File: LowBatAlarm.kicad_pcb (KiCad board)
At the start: 2 copper layers, 30 x 24 mm, 19 parts, among them J1 Battery, J2 Buzzer, Q1 BSN20, U1 ADCMP350, U2 ADP7142AUJZ

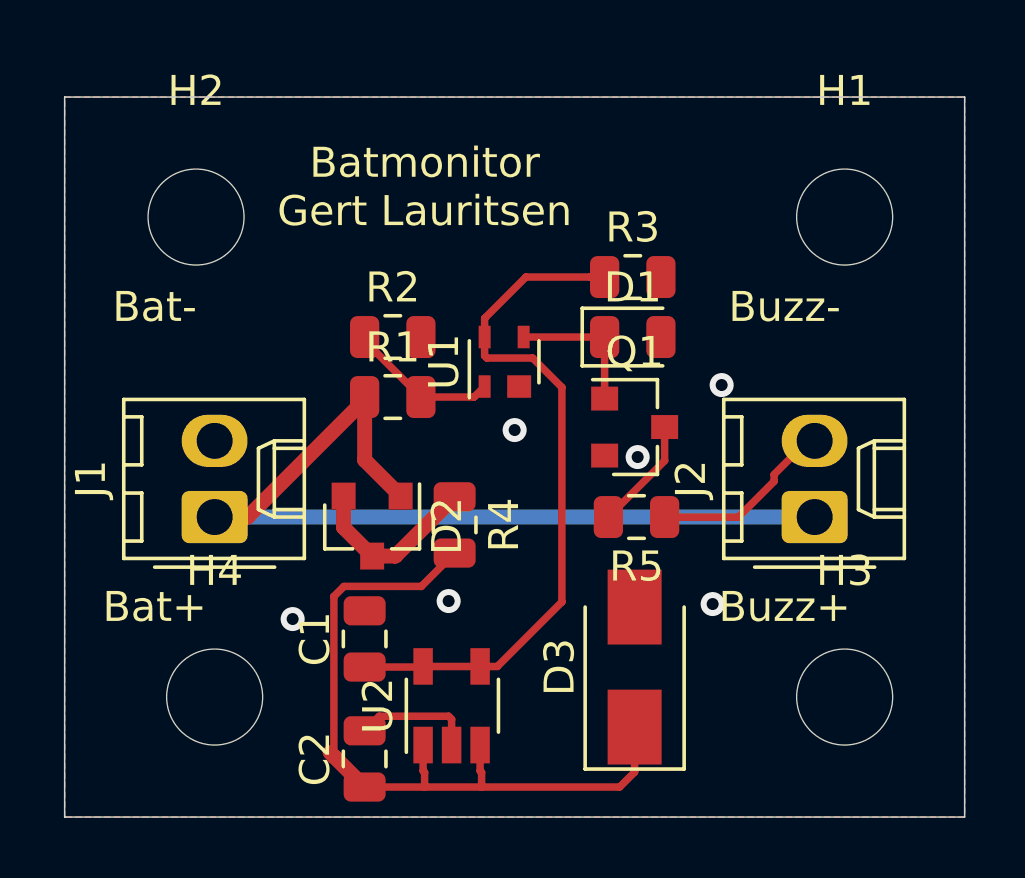
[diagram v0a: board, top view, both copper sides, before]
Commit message: PCB opdatering
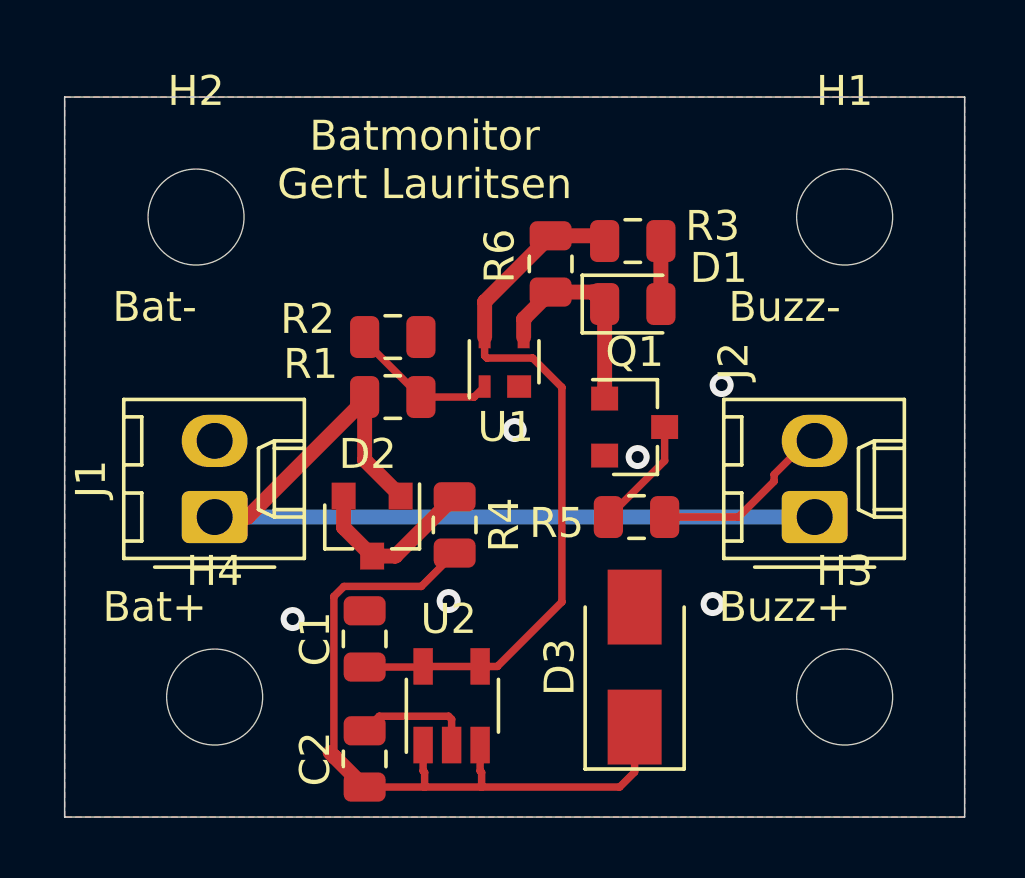
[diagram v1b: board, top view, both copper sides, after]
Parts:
- added R6: 1k, Resistor_SMD:R_0805_2012Metric, F.Cu at (140.2, 91.6)
- R2: value 100k -> TBD
- moved R3 1.20 mm to (142.9, 90.8)
- moved D1 1.10 mm to (142.9, 92.9)
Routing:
- net Net-(D1-Pad1): track 4.75 -> 6.99 mm
- net Net-(D1-Pad2): track 0.00 -> 2.10 mm
- net +3V3: track 23.5 -> 24.4 mm
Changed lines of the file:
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@@
     (thickness 1.6)
     (drawings 11)
-    (tracks 66)
+    (tracks 70)
     (zones 0)
-    (modules 19)
+    (modules 20)
     (nets 11)
   )
@@
   )
   (setup
-    (last_trace_width 0.25)
+    (last_trace_width 0.5)
     (user_trace_width 0.5)
     (trace_clearance 0.2)
@@
     (solder_mask_min_width 0.25)
     (aux_axis_origin 0 0)
-    (visible_elements 7FFFFFFF)
+    (visible_elements 7FF9FFFF)
     (pcbplotparams
       (layerselection 0x010fc_ffffffff)
@@
   )
   (module Resistor_SMD:R_0805_2012Metric (layer F.Cu)
+    (at 140.2 91.5625 270)
+    (descr "Resistor SMD 0805 (2012 Metric), square (rectangular) end terminal, IPC_7351 nominal, (Body size source: https://docs.google.com/spreadsheets/d/1BsfQQcO9C6DZCsRaXUlFlo91Tg2WpOkGARC1WS5S8t0/edit?usp=sharing), generated with kicad-footprint-generator")
+    (tags resistor)
+    (attr smd)
+    (fp_text reference R6 (at -0.2625 1.7 90) (layer F.SilkS)
+      (effects (font (size 1 1) (thickness 0.15)))
+    )
+    (fp_text value 1k (at 0 1.65 90) (layer F.Fab)
+      (effects (font (size 1 1) (thickness 0.15)))
+    )
+    (fp_text user %R (at 0 0 90) (layer F.Fab)
+      (effects (font (size 0.5 0.5) (thickness 0.08)))
+    )
+    (fp_line (start 1.68 0.95) (end -1.68 0.95) (layer F.CrtYd) (width 0.05))
+    (fp_line (start 1.68 -0.95) (end 1.68 0.95) (layer F.CrtYd) (width 0.05))
+    (fp_line (start -1.68 -0.95) (end 1.68 -0.95) (layer F.CrtYd) (width 0.05))
+    (fp_line (start -1.68 0.95) (end -1.68 -0.95) (layer F.CrtYd) (width 0.05))
+    (fp_line (start -0.258578 0.71) (end 0.258578 0.71) (layer F.SilkS) (width 0.12))
+    (fp_line (start -0.258578 -0.71) (end 0.258578 -0.71) (layer F.SilkS) (width 0.12))
+    (fp_line (start 1 0.6) (end -1 0.6) (layer F.Fab) (width 0.1))
+    (fp_line (start 1 -0.6) (end 1 0.6) (layer F.Fab) (width 0.1))
+    (fp_line (start -1 -0.6) (end 1 -0.6) (layer F.Fab) (width 0.1))
+    (fp_line (start -1 0.6) (end -1 -0.6) (layer F.Fab) (width 0.1))
+    (pad 2 smd roundrect (at 0.9375 0 270) (size 0.975 1.4) (layers F.Cu F.Paste F.Mask) (roundrect_rratio 0.25)
+      (net 2 "Net-(D1-Pad1)"))
+    (pad 1 smd roundrect (at -0.9375 0 270) (size 0.975 1.4) (layers F.Cu F.Paste F.Mask) (roundrect_rratio 0.25)
+      (net 7 +3V3))
+    (model ${KISYS3DMOD}/Resistor_SMD.3dshapes/R_0805_2012Metric.wrl
+      (at (xyz 0 0 0))
+      (scale (xyz 1 1 1))
+      (rotate (xyz 0 0 0))
+    )
+  )
+  (module Resistor_SMD:R_0805_2012Metric (layer F.Cu)
     (at 143.0625 100 180)
     (descr "Resistor SMD 0805 (2012 Metric), square (rectangular) end terminal, IPC_7351 nominal, (Body size source: https://docs.google.com/spreadsheets/d/1BsfQQcO9C6DZCsRaXUlFlo91Tg2WpOkGARC1WS5S8t0/edit?usp=sharing), generated with kicad-footprint-generator")
     (tags resistor)
     (attr smd)
-    (fp_text reference R5 (at 0 -1.65) (layer F.SilkS)
+    (fp_text reference R5 (at 2.6625 -0.2) (layer F.SilkS)
       (effects (font (size 1 1) (thickness 0.15)))
     )
@@
     (tags SOT-23)
     (attr smd)
-    (fp_text reference D2 (at 0 -2.5 90) (layer F.SilkS)
+    (fp_text reference D2 (at -2.4 0.15 180) (layer F.SilkS)
       (effects (font (size 1 1) (thickness 0.15)))
     )
@@
     (tags TSOT-23-5)
     (attr smd)
-    (fp_text reference U2 (at 0 -2.45 90) (layer F.SilkS)
+    (fp_text reference U2 (at 2.89 -0.1 180) (layer F.SilkS)
       (effects (font (size 1 1) (thickness 0.15)))
     )
@@
     (tags resistor)
     (attr smd)
-    (fp_text reference R2 (at 0 -1.65) (layer F.SilkS)
-      (effects (font (size 1 1) (thickness 0.15)))
-    )
-    (fp_text value 100k (at 0 1.65) (layer F.Fab)
-      (effects (font (size 1 1) (thickness 0.15)))
-    )
-    (fp_text user %R (at 0 0) (layer F.Fab)
+    (fp_text reference R2 (at -2.8375 -0.6) (layer F.SilkS)
+      (effects (font (size 1 1) (thickness 0.15)))
+    )
+    (fp_text value TBD (at 0 1.65) (layer F.Fab)
+      (effects (font (size 1 1) (thickness 0.15)))
+    )
+    (fp_text user %R (at -2.6375 1.3) (layer F.Fab)
       (effects (font (size 0.5 0.5) (thickness 0.08)))
     )
@@
     (tags resistor)
     (attr smd)
-    (fp_text reference R1 (at 0 -1.65) (layer F.SilkS)
+    (fp_text reference R1 (at -2.7375 -1.1) (layer F.SilkS)
       (effects (font (size 1 1) (thickness 0.15)))
     )
@@
     (tags "Analog Devices KS-4 (like EIAJ SC-82)")
     (attr smd)
-    (fp_text reference U1 (at 0 -2 90) (layer F.SilkS)
+    (fp_text reference U1 (at -2.175 0.05 180) (layer F.SilkS)
       (effects (font (size 1 1) (thickness 0.15)))
     )
@@
   )
   (module Resistor_SMD:R_0805_2012Metric (layer F.Cu)
-    (at 142.9375 92)
+    (at 142.9375 90.8)
     (descr "Resistor SMD 0805 (2012 Metric), square (rectangular) end terminal, IPC_7351 nominal, (Body size source: https://docs.google.com/spreadsheets/d/1BsfQQcO9C6DZCsRaXUlFlo91Tg2WpOkGARC1WS5S8t0/edit?usp=sharing), generated with kicad-footprint-generator")
     (tags resistor)
     (attr smd)
-    (fp_text reference R3 (at 0 -1.65) (layer F.SilkS)
+    (fp_text reference R3 (at 2.6625 -0.5) (layer F.SilkS)
       (effects (font (size 1 1) (thickness 0.15)))
     )
@@
     (descr "Molex KK-254 Interconnect System, old/engineering part number: AE-6410-02A example for new part number: 22-27-2021, 2 Pins (http://www.molex.com/pdm_docs/sd/022272021_sd.pdf), generated with kicad-footprint-generator")
     (tags "connector Molex KK-254 side entry")
-    (fp_text reference J2 (at 1.27 -4.12 90) (layer F.SilkS)
+    (fp_text reference J2 (at 5.2 -2.7 90) (layer F.SilkS)
       (effects (font (size 1 1) (thickness 0.15)))
     )
@@
   )
   (module LED_SMD:LED_0805_2012Metric (layer F.Cu)
-    (at 142.9375 94)
+    (at 142.9375 92.9)
     (descr "LED SMD 0805 (2012 Metric), square (rectangular) end terminal, IPC_7351 nominal, (Body size source: https://docs.google.com/spreadsheets/d/1BsfQQcO9C6DZCsRaXUlFlo91Tg2WpOkGARC1WS5S8t0/edit?usp=sharing), generated with kicad-footprint-generator")
     (tags diode)
     (attr smd)
-    (fp_text reference D1 (at 0 -1.65) (layer F.SilkS)
+    (fp_text reference D1 (at 2.8625 -1.2) (layer F.SilkS)
       (effects (font (size 1 1) (thickness 0.15)))
     )
@@
     (effects (font (size 1 1) (thickness 0.15)))
   )
-  (gr_text "Batmonitor\nGert Lauritsen" (at 136 89) (layer F.SilkS)
+  (gr_text "Batmonitor\nGert Lauritsen" (at 136 88.1) (layer F.SilkS)
     (effects (font (size 1 1) (thickness 0.15)))
   )
@@
   (gr_line (start 154 86) (end 154 110) (layer Edge.Cuts) (width 0.05))
   (gr_line (start 124 86) (end 154 86) (layer Edge.Cuts) (width 0.05))
-  (segment (start 139.3 94) (end 142 94) (width 0.25) (layer F.Cu) (net 2))
-  (segment (start 142 96.05) (end 142 94) (width 0.25) (layer F.Cu) (net 2))
+  (segment (start 143.875 90.8) (end 143.875 92.9) (width 0.5) (layer F.Cu) (net 1))
+  (segment (start 141.6 92.5) (end 142 92.9) (width 0.5) (layer F.Cu) (net 2))
+  (segment (start 140.2 92.5) (end 141.6 92.5) (width 0.5) (layer F.Cu) (net 2))
+  (segment (start 139.3 93.4) (end 140.2 92.5) (width 0.5) (layer F.Cu) (net 2))
+  (segment (start 139.3 94) (end 139.3 93.4) (width 0.5) (layer F.Cu) (net 2))
+  (segment (start 142 96.05) (end 142 92.9) (width 0.5) (layer F.Cu) (net 2))
   (segment (start 136.799473 106.639473) (end 134.485527 106.639473) (width 0.25) (layer F.Cu) (net 3))
   (segment (start 134.485527 106.639473) (end 134 107.125) (width 0.25) (layer F.Cu) (net 3))
@@
   (segment (start 137.65 96) (end 138 95.65) (width 0.25) (layer F.Cu) (net 6))
   (segment (start 135.875 96) (end 137.65 96) (width 0.25) (layer F.Cu) (net 6))
-  (segment (start 139.375 92) (end 141.5125 92) (width 0.25) (layer F.Cu) (net 7))
-  (segment (start 141.5125 92) (end 142 92) (width 0.25) (layer F.Cu) (net 7))
-  (segment (start 138 93.375) (end 139.375 92) (width 0.25) (layer F.Cu) (net 7))
-  (segment (start 138 94) (end 138 93.375) (width 0.25) (layer F.Cu) (net 7))
   (segment (start 135.93 105) (end 135.95 104.98) (width 0.25) (layer F.Cu) (net 7))
   (segment (start 134 105) (end 135.93 105) (width 0.25) (layer F.Cu) (net 7))
@@
   (segment (start 138.075001 94.700001) (end 138 94.625) (width 0.25) (layer F.Cu) (net 7))
   (segment (start 137.85 104.98) (end 138.425 104.98) (width 0.25) (layer F.Cu) (net 7))
+  (segment (start 141.825 90.625) (end 142 90.8) (width 0.5) (layer F.Cu) (net 7))
+  (segment (start 140.2 90.625) (end 141.825 90.625) (width 0.5) (layer F.Cu) (net 7))
+  (segment (start 138 92.825) (end 138 94) (width 0.5) (layer F.Cu) (net 7))
+  (segment (start 140.2 90.625) (end 138 92.825) (width 0.5) (layer F.Cu) (net 7))
   (segment (start 132.97499 107.97499) (end 133 108) (width 0.25) (layer F.Cu) (net 8))
   (segment (start 132.97499 102.64566) (end 132.97499 107.97499) (width 0.25) (layer F.Cu) (net 8))
